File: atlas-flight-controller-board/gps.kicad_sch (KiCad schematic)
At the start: 1 part, among them U2 MAX-M10S-00B

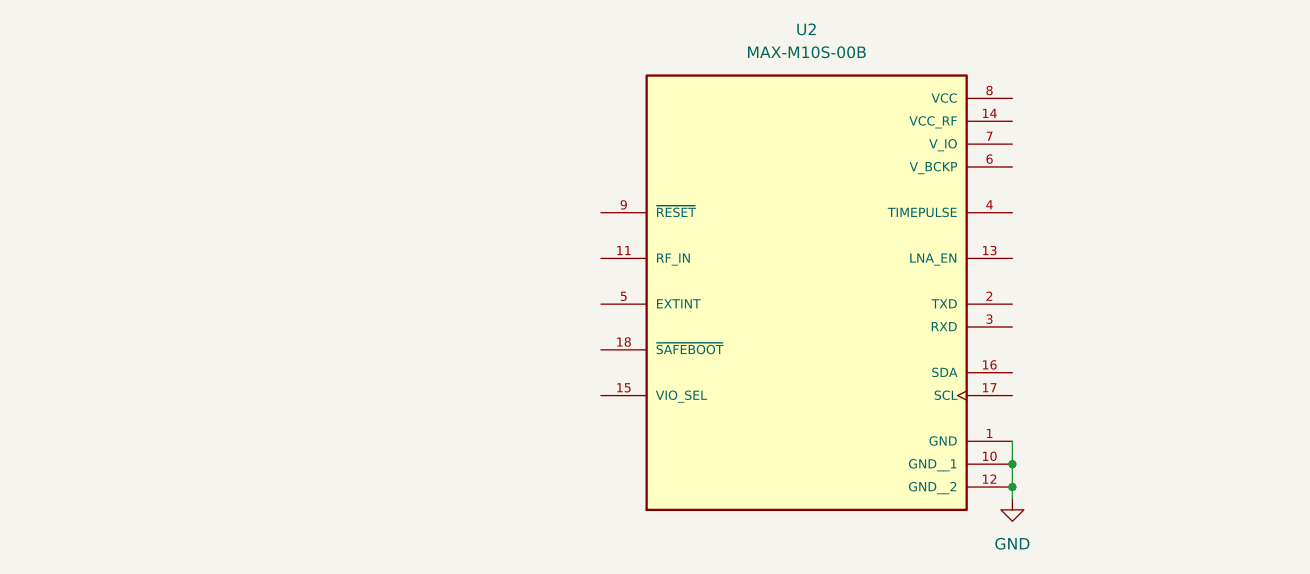
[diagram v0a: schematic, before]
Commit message: finishing up schematic for v1.
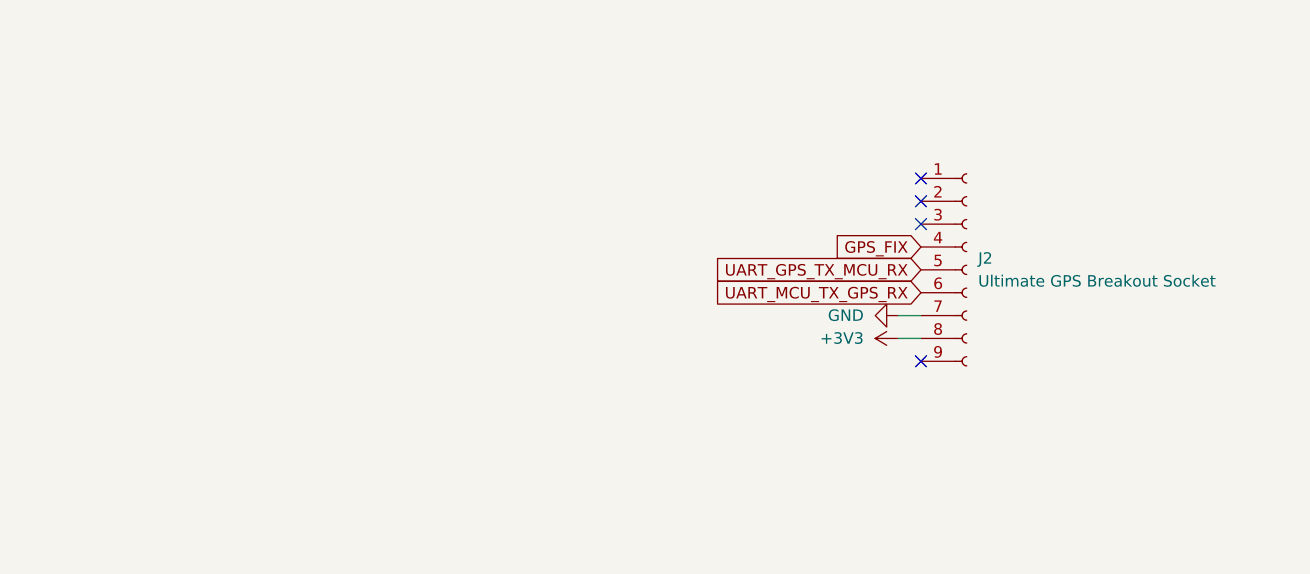
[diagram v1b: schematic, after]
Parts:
- removed U2: MAX-M10S-00B, MAX_M10S_00B:XCVR_MAX-M10S-00B, symbol MAX-M10S-00B:MAX-M10S-00B
- added J2: Ultimate GPS Breakout Socket, Connector_PinHeader_2.54mm:PinHeader_1x09_P2.54mm_Vertical, symbol Connector:Conn_01x09_Socket
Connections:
- net GND: now also J2.7 (Pin_7)
- new net +3V3: J2.8 (Pin_8)
- new net GPS_FIX: J2.4 (Pin_4)
- new net UART_GPS_TX_MCU_RX: J2.5 (Pin_5)
- new net UART_MCU_TX_GPS_RX: J2.6 (Pin_6)
- no-connect marks 0 -> 4
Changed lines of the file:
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@@
 	(generator_version "9.0")
 	(paper "A4")
-	(junction
-		(at 139.7 115.57)
-		(diameter 0)
-		(color 0 0 0 0)
-	)
-	(junction
-		(at 139.7 113.03)
-		(diameter 0)
-		(color 0 0 0 0)
+	(no_connect
+		(at 129.54 101.6)
+	)
+	(no_connect
+		(at 129.54 83.82)
+	)
+	(no_connect
+		(at 129.54 81.28)
+	)
+	(no_connect
+		(at 129.54 86.36)
 	)
 	(wire
 		(pts
-			(xy 139.7 115.57) (xy 139.7 116.84)
+			(xy 127 96.52) (xy 129.54 96.52)
 		)
 		(stroke
@@
 	(wire
 		(pts
-			(xy 139.7 113.03) (xy 139.7 115.57)
+			(xy 127 99.06) (xy 129.54 99.06)
 		)
 		(stroke
@@
 		)
 	)
-	(wire
-		(pts
-			(xy 139.7 110.49) (xy 139.7 113.03)
-		)
-		(stroke
-			(width 0)
-			(type default)
+	(global_label "GPS_FIX"
+		(shape input)
+		(at 129.54 88.9 180)
+		(fields_autoplaced yes)
+		(effects
+			(font
+				(size 1.27 1.27)
+			)
+			(justify right)
+		)
+		(property "Intersheetrefs" "${INTERSHEET_REFS}"
+			(at 118.9348 88.9 0)
+			(effects
+				(font
+					(size 1.27 1.27)
+				)
+				(justify right)
+				(hide yes)
+			)
+		)
+	)
+	(global_label "UART_GPS_TX_MCU_RX"
+		(shape input)
+		(at 129.54 91.44 180)
+		(fields_autoplaced yes)
+		(effects
+			(font
+				(size 1.27 1.27)
+			)
+			(justify right)
+		)
+		(property "Intersheetrefs" "${INTERSHEET_REFS}"
+			(at 105.5697 91.44 0)
+			(effects
+				(font
+					(size 1.27 1.27)
+				)
+				(justify right)
+				(hide yes)
+			)
+		)
+	)
+	(global_label "UART_MCU_TX_GPS_RX"
+		(shape input)
+		(at 129.54 93.98 180)
+		(fields_autoplaced yes)
+		(effects
+			(font
+				(size 1.27 1.27)
+			)
+			(justify right)
+		)
+		(property "Intersheetrefs" "${INTERSHEET_REFS}"
+			(at 105.5697 93.98 0)
+			(effects
+				(font
+					(size 1.27 1.27)
+				)
+				(justify right)
+				(hide yes)
+			)
 		)
 	)
 	(symbol
-		(lib_id "MAX-M10S-00B:MAX-M10S-00B")
-		(at 116.84 90.17 0)
+		(lib_id "power:GND")
+		(at 127 96.52 270)
 		(unit 1)
 		(exclude_from_sim no)
@@
 		(dnp no)
 		(fields_autoplaced yes)
-		(property "Reference" "U2"
-			(at 116.84 64.77 0)
-			(effects
-				(font
-					(size 1.27 1.27)
-				)
-			)
-		)
-		(property "Value" "MAX-M10S-00B"
-			(at 116.84 67.31 0)
-			(effects
-				(font
-					(size 1.27 1.27)
-				)
-			)
-		)
-		(property "Footprint" "MAX_M10S_00B:XCVR_MAX-M10S-00B"
-			(at 116.84 90.17 0)
-			(effects
-				(font
-					(size 1.27 1.27)
-				)
-				(justify bottom)
+		(property "Reference" "#PWR03"
+			(at 120.65 96.52 0)
+			(effects
+				(font
+					(size 1.27 1.27)
+				)
+				(hide yes)
+			)
+		)
+		(property "Value" "GND"
+			(at 123.19 96.5199 90)
+			(effects
+				(font
+					(size 1.27 1.27)
+				)
+				(justify right)
+			)
+		)
+		(property "Footprint" ""
+			(at 127 96.52 0)
+			(effects
+				(font
+					(size 1.27 1.27)
+				)
 				(hide yes)
 			)
 		)
 		(property "Datasheet" ""
-			(at 116.84 90.17 0)
-			(effects
-				(font
-					(size 1.27 1.27)
-				)
-				(hide yes)
-			)
-		)
-		(property "Description" ""
-			(at 116.84 90.17 0)
-			(effects
-				(font
-					(size 1.27 1.27)
-				)
-				(hide yes)
-			)
-		)
-		(property "PARTREV" "C1"
-			(at 116.84 90.17 0)
-			(effects
-				(font
-					(size 1.27 1.27)
-				)
-				(justify bottom)
-				(hide yes)
-			)
-		)
-		(property "STANDARD" "Manufacturer Recommendations"
-			(at 116.84 90.17 0)
-			(effects
-				(font
-					(size 1.27 1.27)
-				)
-				(justify bottom)
-				(hide yes)
-			)
-		)
-		(property "MAXIMUM_PACKAGE_HEIGHT" "2.7mm"
-			(at 116.84 90.17 0)
-			(effects
-				(font
-					(size 1.27 1.27)
-				)
-				(justify bottom)
-				(hide yes)
-			)
-		)
-		(property "MANUFACTURER" "u-blox"
-			(at 116.84 90.17 0)
-			(effects
-				(font
-					(size 1.27 1.27)
-				)
-				(justify bottom)
-				(hide yes)
-			)
-		)
-		(pin "5"
-		)
-		(pin "18"
-		)
-		(pin "14"
-		)
-		(pin "16"
-		)
-		(pin "15"
-		)
-		(pin "17"
+			(at 127 96.52 0)
+			(effects
+				(font
+					(size 1.27 1.27)
+				)
+				(hide yes)
+			)
+		)
+		(property "Description" "Power symbol creates a global label with name \"GND\" , ground"
+			(at 127 96.52 0)
+			(effects
+				(font
+					(size 1.27 1.27)
+				)
+				(hide yes)
+			)
 		)
 		(pin "1"
-		)
-		(pin "2"
-		)
-		(pin "11"
-		)
-		(pin "10"
-		)
-		(pin "8"
-		)
-		(pin "4"
-		)
-		(pin "7"
-		)
-		(pin "13"
-		)
-		(pin "3"
-		)
-		(pin "6"
-		)
-		(pin "12"
-		)
-		(pin "9"
 		)
 		(instances
 			(project ""
 				(path "/99efb2d6-b5f7-438c-9ed2-f359400f01a1/b614d0fa-38cc-4f5c-8335-684f0616169f"
-					(reference "U2")
+					(reference "#PWR03")
 					(unit 1)
 				)
@@
 	)
 	(symbol
-		(lib_id "power:GND")
-		(at 139.7 116.84 0)
+		(lib_id "Connector:Conn_01x09_Socket")
+		(at 134.62 91.44 0)
 		(unit 1)
 		(exclude_from_sim no)
@@
 		(dnp no)
 		(fields_autoplaced yes)
-		(property "Reference" "#PWR016"
-			(at 139.7 123.19 0)
-			(effects
-				(font
-					(size 1.27 1.27)
-				)
-				(hide yes)
-			)
-		)
-		(property "Value" "GND"
-			(at 139.7 121.92 0)
-			(effects
-				(font
-					(size 1.27 1.27)
-				)
-			)
-		)
-		(property "Footprint" ""
-			(at 139.7 116.84 0)
-			(effects
-				(font
-					(size 1.27 1.27)
-				)
-				(hide yes)
-			)
-		)
-		(property "Datasheet" ""
-			(at 139.7 116.84 0)
-			(effects
-				(font
-					(size 1.27 1.27)
-				)
-				(hide yes)
-			)
-		)
-		(property "Description" "Power symbol creates a global label with name \"GND\" , ground"
-			(at 139.7 116.84 0)
-			(effects
-				(font
-					(size 1.27 1.27)
-				)
-				(hide yes)
-			)
+		(property "Reference" "J2"
+			(at 135.89 90.1699 0)
+			(effects
+				(font
+					(size 1.27 1.27)
+				)
+				(justify left)
+			)
+		)
+		(property "Value" "Ultimate GPS Breakout Socket"
+			(at 135.89 92.7099 0)
+			(effects
+				(font
+					(size 1.27 1.27)
+				)
+				(justify left)
+			)
+		)
+		(property "Footprint" "Connector_PinHeader_2.54mm:PinHeader_1x09_P2.54mm_Vertical"
+			(at 134.62 91.44 0)
+			(effects
+				(font
+					(size 1.27 1.27)
+				)
+				(hide yes)
+			)
+		)
+		(property "Datasheet" "~"
+			(at 134.62 91.44 0)
+			(effects
+				(font
+					(size 1.27 1.27)
+				)
+				(hide yes)
+			)
+		)
+		(property "Description" "Generic connector, single row, 01x09, script generated"
+			(at 134.62 91.44 0)
+			(effects
+				(font
+					(size 1.27 1.27)
+				)
+				(hide yes)
+			)
+		)
+		(pin "8"
+		)
+		(pin "9"
+		)
+		(pin "4"
+		)
+		(pin "7"
+		)
+		(pin "6"
+		)
+		(pin "5"
+		)
+		(pin "3"
+		)
+		(pin "2"
 		)
 		(pin "1"
@@
 			(project ""
 				(path "/99efb2d6-b5f7-438c-9ed2-f359400f01a1/b614d0fa-38cc-4f5c-8335-684f0616169f"
-					(reference "#PWR016")
+					(reference "J2")
 					(unit 1)
 				)
+			)
+		)
+	)
+	(symbol
+		(lib_id "power:+3V3")
+		(at 127 99.06 90)
+		(unit 1)
+		(exclude_from_sim no)
+		(in_bom yes)
+		(on_board yes)
+		(dnp no)
+		(fields_autoplaced yes)
+		(property "Reference" "#PWR04"
+			(at 130.81 99.06 0)
+			(effects
+				(font
+					(size 1.27 1.27)
+				)
+				(hide yes)
+			)
+		)
+		(property "Value" "+3V3"
+			(at 123.19 99.0599 90)
+			(effects
+				(font
+					(size 1.27 1.27)
+				)
+				(justify left)
+			)
+		)
+		(property "Footprint" ""
+			(at 127 99.06 0)
+			(effects
+				(font
+					(size 1.27 1.27)
+				)
+				(hide yes)
+			)
+		)
+		(property "Datasheet" ""
+			(at 127 99.06 0)
+			(effects
+				(font
+					(size 1.27 1.27)
+				)
+				(hide yes)
+			)
+		)
+		(property "Description" "Power symbol creates a global label with name \"+3V3\""
+			(at 127 99.06 0)
+			(effects
+				(font
+					(size 1.27 1.27)
+				)
+				(hide yes)
+			)
+		)
+		(pin "1"
+		)
+		(instances
+			(project ""
+				(path "/99efb2d6-b5f7-438c-9ed2-f359400f01a1/b614d0fa-38cc-4f5c-8335-684f0616169f"
+					(reference "#PWR04")
+					(unit 1)
+				)

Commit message: Done.
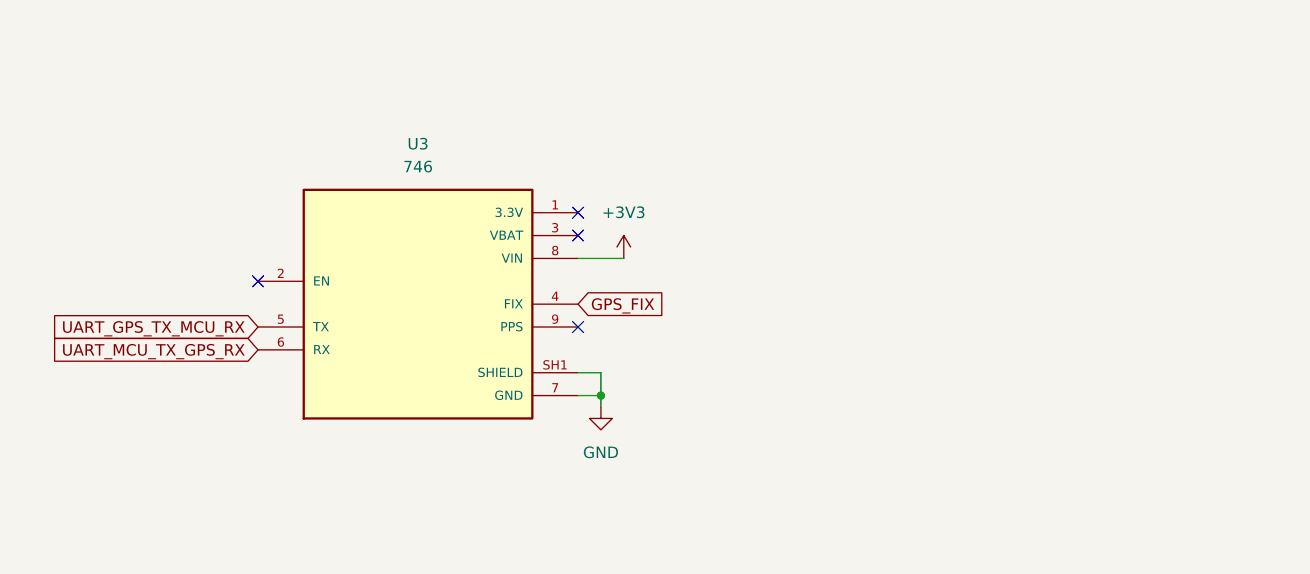
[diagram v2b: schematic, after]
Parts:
- removed J2: Ultimate GPS Breakout Socket, Connector_PinHeader_2.54mm:PinHeader_1x09_P2.54mm_Vertical, symbol Connector:Conn_01x09_Socket
- added U3: 746, 746:XCVR_746, symbol Ultimate-gps-v3:746
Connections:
- net +3V3: now also U3.8 (VIN)
- net GND: now also U3.7 (GND), U3.SH1 (SHIELD), U3.SH2 (SHIELD)
- net GPS_FIX: now also U3.4 (FIX)
- net UART_GPS_TX_MCU_RX: now also U3.5 (TX)
- net UART_MCU_TX_GPS_RX: now also U3.6 (RX)
